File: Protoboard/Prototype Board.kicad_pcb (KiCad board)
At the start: 2 copper layers, 99.1 x 99.1 mm, 433 parts, among them J1 Conn_01x01, J10 Conn_01x01, J100 Connectable_Pad_Group_01x04, J101 Connectable_Pad_Group_01x04, J102 Connectable_Pad_Group_01x04, J103 Connectable_Pad_Group_01x04, J104 Connectable_Pad_Group_01x04, J105 Connectable_Pad_Group_01x04, J106 Connectable_Pad_Group_01x04, J107 Connectable_Pad_Group_01x04, J108 Connectable_Pad_Group_01x04, J109 Connectable_Pad_Group_01x04, J11 Conn_01x01, J110 Connectable_Pad_Group_01x04, J111 Connectable_Pad_Group_01x04, J112 Connectable_Pad_Group_01x04, J113 Connectable_Pad_Group_01x04, J114 Connectable_Pad_Group_01x04, J115 Connectable_Pad_Group_01x04, J116 Connectable_Pad_Group_01x04, J117 Connectable_Pad_Group_01x04, J118 Connectable_Pad_Group_01x04, J119 Connectable_Pad_Group_01x04, J12 Conn_01x01, J120 Connectable_Pad_Group_01x04, J121 Connectable_Pad_Group_01x04, J122 Connectable_Pad_Group_01x04, J123 Connectable_Pad_Group_01x04, J124 Connectable_Pad_Group_01x04, J125 Connectable_Pad_Group_01x04, J126 Connectable_Pad_Group_01x04, J13 Conn_01x01, J133 Conn_01x03_Male, J134 Conn_01x03_Male, J135 Connectable_Pad_Group_01x04, J136 Connectable_Pad_Group_01x04, J137 Connectable_Pad_Group_01x04, J138 Connectable_Pad_Group_01x04, J139 Connectable_Pad_Group_01x04, J14 Conn_01x01, J140 Connectable_Pad_Group_01x04, J141 Connectable_Pad_Group_01x04, J142 Connectable_Pad_Group_01x04, J143 Connectable_Pad_Group_01x04, J144 Connectable_Pad_Group_01x04, J145 Connectable_Pad_Group_01x04, J146 Connectable_Pad_Group_01x04, J147 Connectable_Pad_Group_01x04, J148 Connectable_Pad_Group_01x04, J149 Connectable_Pad_Group_01x04, J15 Conn_01x01, J150 Connectable_Pad_Group_01x04, J151 Connectable_Pad_Group_01x04, J152 Connectable_Pad_Group_01x04, J153 Connectable_Pad_Group_01x04, J154 Connectable_Pad_Group_01x04, J155 Connectable_Pad_Group_01x04, J156 Connectable_Pad_Group_01x04, J157 Connectable_Pad_Group_01x04, J158 Connectable_Pad_Group_01x04, J159 Connectable_Pad_Group_01x04, J16 Conn_01x01, J160 Connectable_Pad_Group_01x04, J161 Connectable_Pad_Group_01x04, J162 Connectable_Pad_Group_01x04, J163 Connectable_Pad_Group_01x04, J164 Connectable_Pad_Group_01x04, J165 Conn_01x03_Male, J166 Conn_01x03_Male, J17 Connectable_Pad_Group_01x04, J18 Connectable_Pad_Group_01x04, J19 Connectable_Pad_Group_01x04, J2 Conn_01x01, J20 Connectable_Pad_Group_01x04, J21 Connectable_Pad_Group_01x04, J22 Connectable_Pad_Group_01x04, J23 Connectable_Pad_Group_01x04, J24 Connectable_Pad_Group_01x04, J25 Connectable_Pad_Group_01x04, J26 Connectable_Pad_Group_01x04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

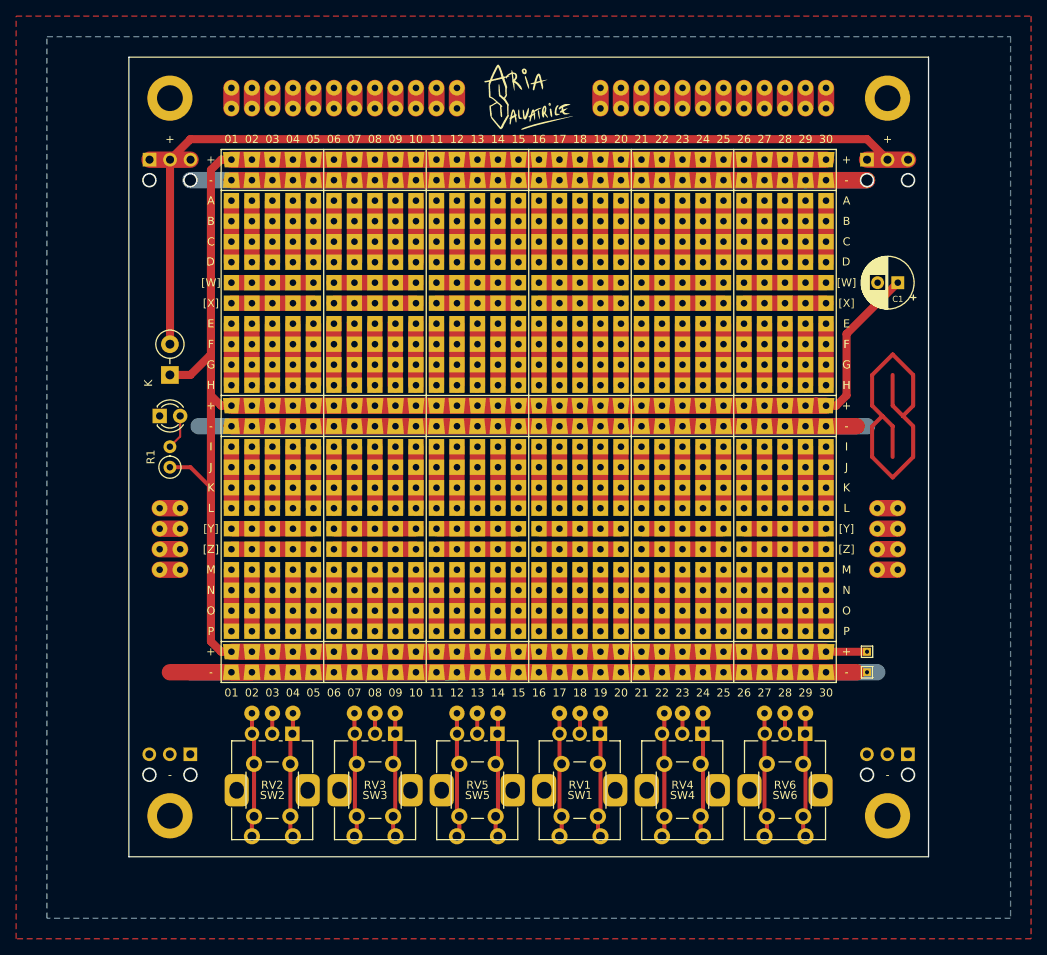
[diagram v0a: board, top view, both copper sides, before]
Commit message: Protoboard Rev2 ready soon, needs checking
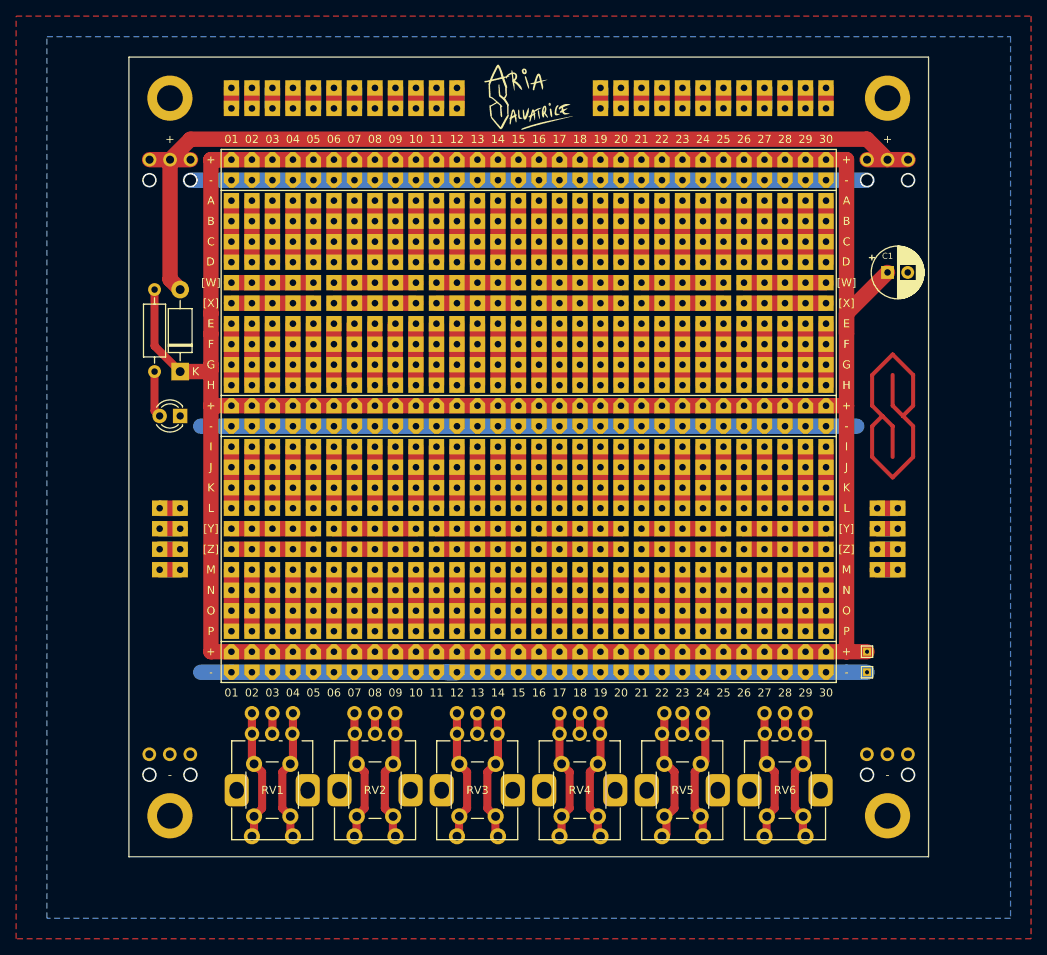
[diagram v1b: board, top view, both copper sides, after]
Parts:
- removed the J167 at (170.2, 43.2)
- removed J168, J169, J170, J171, J172, J173, J193, J194, J195, J196, J197, J198, J214, J215, J216, J217, J218, J219, J220, J221, J222, J223, J224, J225, J226, J227, J228, J229, J230, J231, J232, J233, J234, J235, J236, J237, J238, J239, J240, J241, J242, J243, J244, J245, J246, J247, J248, J249, J250, J251, J252, J253, J254, J255, J256, J257, J258, J259, J260, J261, J262, J263, J264, J265, J266, J267, J268, J269, J270, J271, J272, J273, J274, J275, J276, J277, J278, J279, J280, J281, J282, J283, J284, J285, J286, J287, J288, J289, J290, J291, J292, J293, J294, J295, J296, J297, J298, J299, J300, J301, J302, J303, J304, J305, J306, J307, J308, J309, J310, J311, J312, J313, J314, J315, J316, J317, J318, J319, J320, J321, J322, J323, J324, J325, J326, J327, J328, J329, J330, J331, J332, J333, J334, J335, J336, J337, J338, J339, J340, J341, J342, J343, J344, J345, J346: ~, ao_tht:Perf_Board_Hole
- removed the J174 at (167.6, 43.2)
- removed the J175 at (127.0, 43.2)
- removed the J176 at (142.2, 43.2)
- removed the J177 at (114.3, 43.2)
- removed the J178 at (116.8, 43.2)
- removed the J179 at (149.9, 43.2)
- removed the J180 at (106.7, 43.2)
- removed the J181 at (147.3, 43.2)
- removed the J182 at (172.7, 43.2)
- removed the J183 at (154.9, 43.2)
- removed the J184 at (124.5, 43.2)
- removed the J185 at (119.4, 43.2)
- removed the J186 at (144.8, 43.2)
- removed the J187 at (109.2, 43.2)
- removed the J188 at (152.4, 43.2)
- removed the J189 at (139.7, 43.2)
- removed the J190 at (162.6, 43.2)
- removed the J191 at (132.1, 43.2)
- removed the J192 at (160.0, 43.2)
- removed the J199 at (165.1, 45.7)
- removed the J200 at (137.2, 45.7)
- removed the J201 at (116.8, 45.7)
- removed the J202 at (144.8, 45.7)
- removed the J203 at (127.0, 45.7)
- removed the J204 at (157.5, 45.7)
- removed the J205 at (149.9, 45.7)
- removed the J206 at (124.5, 45.7)
- removed the J207 at (114.3, 45.7)
- removed the J208 at (175.3, 45.7)
- removed the J209 at (104.1, 45.7)
- removed the J210 at (139.7, 45.7)
- removed the J211 at (106.7, 45.7)
- removed the J212 at (160.0, 45.7)
- removed the J213 at (109.2, 45.7)
- removed the REF** at (177.8, 34.3)
- removed the REF** at (132.1, 34.3)
- removed the REF** at (95.2, 91.4)
- removed the REF** at (121.9, 36.8)
- removed the REF** at (152.4, 34.3)
- removed the REF** at (184.2, 94.0)
- removed the REF** at (97.8, 91.4)
- removed the REF** at (167.6, 36.8)
- removed the REF** at (97.8, 94.0)
- removed the REF** at (152.4, 36.8)
- removed the REF** at (114.3, 34.3)
- removed the REF** at (160.0, 34.3)
- removed the REF** at (184.2, 88.9)
- removed the REF** at (175.3, 36.8)
- removed the REF** at (172.7, 34.3)
- removed the REF** at (95.2, 86.4)
- removed the REF** at (170.2, 34.3)
- removed the REF** at (129.5, 34.3)
- removed the REF** at (175.3, 34.3)
- removed the REF** at (154.9, 34.3)
- removed the REF** at (109.2, 34.3)
- removed the REF** at (111.8, 34.3)
- removed the REF** at (119.4, 34.3)
- removed the REF** at (116.8, 34.3)
- removed the REF** at (165.1, 36.8)
- removed the REF** at (184.2, 91.4)
- removed the REF** at (119.4, 36.8)
- removed the REF** at (157.5, 36.8)
- removed the REF** at (160.0, 36.8)
- removed the REF** at (186.7, 94.0)
- removed the REF** at (170.2, 36.8)
- removed the REF** at (154.9, 36.8)
- removed the REF** at (132.1, 36.8)
- removed the REF** at (124.5, 36.8)
- removed the REF** at (95.2, 88.9)
- removed the REF** at (127.0, 36.8)
- removed the REF** at (172.7, 36.8)
- removed the REF** at (149.9, 34.3)
- removed the REF** at (111.8, 36.8)
- removed the REF** at (186.7, 91.4)
- removed the REF** at (97.8, 86.4)
- removed the REF** at (106.7, 34.3)
- removed the REF** at (129.5, 36.8)
- removed the REF** at (177.8, 36.8)
- removed the REF** at (186.7, 86.4)
- removed the REF** at (116.8, 36.8)
- removed the REF** at (97.8, 88.9)
- removed the REF** at (186.7, 88.9)
- removed the REF** at (104.1, 34.3)
- removed the REF** at (109.2, 36.8)
- removed the REF** at (124.5, 34.3)
- removed the REF** at (106.7, 36.8)
- removed the REF** at (167.6, 34.3)
- removed the REF** at (104.1, 36.8)
- removed the REF** at (95.2, 94.0)
- removed the REF** at (121.9, 34.3)
- removed the REF** at (127.0, 34.3)
- removed the REF** at (114.3, 36.8)
- removed the REF** at (157.5, 34.3)
- removed the REF** at (184.2, 86.4)
- removed the REF** at (162.6, 34.3)
- removed the REF** at (165.1, 34.3)
- removed the REF** at (149.9, 36.8)
- removed the REF** at (162.6, 36.8)
- added J1: Connectable_Pad_Group_01x02, Protoboard:Connectable_Pad_Group_01x02, F.Cu at (97.8, 86.4)
- added J103: Connectable_Pad_Group_01x02, Protoboard:Connectable_Pad_Group_01x02, F.Cu at (157.5, 34.3)
- added J11: Power_Rail_30, Protoboard:Power_Rail_30, F.Cu at (104.1, 43.2)
- added J112: Connectable_Pad_Group_01x02, Protoboard:Connectable_Pad_Group_01x02, F.Cu at (160.0, 34.3)
- added J113: Connectable_Pad_Group_01x02, Protoboard:Connectable_Pad_Group_01x02, F.Cu at (162.6, 34.3)
- added J124: Connectable_Pad_Group_01x02, Protoboard:Connectable_Pad_Group_01x02, F.Cu at (165.1, 34.3)
- added J129: Connectable_Pad_Group_01x02, Protoboard:Connectable_Pad_Group_01x02, F.Cu at (167.6, 34.3)
- added J13: Power_Rail_30, Protoboard:Power_Rail_30, F.Cu at (104.1, 73.7)
- added J134: Connectable_Pad_Group_01x02, Protoboard:Connectable_Pad_Group_01x02, F.Cu at (170.2, 34.3)
- added J139: Connectable_Pad_Group_01x02, Protoboard:Connectable_Pad_Group_01x02, F.Cu at (172.7, 34.3)
- added J146: Connectable_Pad_Group_01x02, Protoboard:Connectable_Pad_Group_01x02, F.Cu at (175.3, 34.3)
- added J15: Power_Rail_30, Protoboard:Power_Rail_30, F.Cu at (104.1, 104.1)
- added J151: Connectable_Pad_Group_01x02, Protoboard:Connectable_Pad_Group_01x02, F.Cu at (186.7, 86.4)
- added J152: Connectable_Pad_Group_01x02, Protoboard:Connectable_Pad_Group_01x02, F.Cu at (186.7, 88.9)
- added J153: Connectable_Pad_Group_01x02, Protoboard:Connectable_Pad_Group_01x02, F.Cu at (186.7, 91.4)
- added J154: Connectable_Pad_Group_01x02, Protoboard:Connectable_Pad_Group_01x02, F.Cu at (186.7, 94.0)
- added J159: Connectable_Pad_Group_01x02, Protoboard:Connectable_Pad_Group_01x02, F.Cu at (177.8, 34.3)
- added J16: Connectable_Pad_Group_01x02, Protoboard:Connectable_Pad_Group_01x02, F.Cu at (109.2, 34.3)
- added J2: Connectable_Pad_Group_01x02, Protoboard:Connectable_Pad_Group_01x02, F.Cu at (97.8, 88.9)
- added J25: Connectable_Pad_Group_01x02, Protoboard:Connectable_Pad_Group_01x02, F.Cu at (111.8, 34.3)
- added J3: Connectable_Pad_Group_01x02, Protoboard:Connectable_Pad_Group_01x02, F.Cu at (97.8, 91.4)
- added J30: Connectable_Pad_Group_01x02, Protoboard:Connectable_Pad_Group_01x02, F.Cu at (114.3, 34.3)
- added J35: Connectable_Pad_Group_01x02, Protoboard:Connectable_Pad_Group_01x02, F.Cu at (116.8, 34.3)
- added J4: Connectable_Pad_Group_01x02, Protoboard:Connectable_Pad_Group_01x02, F.Cu at (97.8, 94.0)
- added J42: Connectable_Pad_Group_01x02, Protoboard:Connectable_Pad_Group_01x02, F.Cu at (119.4, 34.3)
- added J47: Connectable_Pad_Group_01x02, Protoboard:Connectable_Pad_Group_01x02, F.Cu at (121.9, 34.3)
- added J5: Connectable_Pad_Group_01x02, Protoboard:Connectable_Pad_Group_01x02, F.Cu at (104.1, 34.3)
- added J56: Connectable_Pad_Group_01x02, Protoboard:Connectable_Pad_Group_01x02, F.Cu at (124.5, 34.3)
- added J6: Connectable_Pad_Group_01x02, Protoboard:Connectable_Pad_Group_01x02, F.Cu at (106.7, 34.3)
- added J61: Connectable_Pad_Group_01x02, Protoboard:Connectable_Pad_Group_01x02, F.Cu at (127.0, 34.3)
- added J62: Connectable_Pad_Group_01x02, Protoboard:Connectable_Pad_Group_01x02, F.Cu at (129.5, 34.3)
- added J73: Connectable_Pad_Group_01x02, Protoboard:Connectable_Pad_Group_01x02, F.Cu at (132.1, 34.3)
- added J86: Connectable_Pad_Group_01x02, Protoboard:Connectable_Pad_Group_01x02, F.Cu at (149.9, 34.3)
- added J91: Connectable_Pad_Group_01x02, Protoboard:Connectable_Pad_Group_01x02, F.Cu at (152.4, 34.3)
- added J98: Connectable_Pad_Group_01x02, Protoboard:Connectable_Pad_Group_01x02, F.Cu at (154.9, 34.3)
- D1: footprint Diode_THT:D_DO-41_SOD81_P3.81mm_Vertical_KathodeUp -> Diode_THT:D_DO-41_SOD81_P10.16mm_Horizontal
- R1: value 1K -> 4K7; footprint Resistor_THT:R_Axial_DIN0207_L6.3mm_D2.5mm_P2.54mm_Vertical -> Resistor_THT:R_Axial_DIN0207_L6.3mm_D2.5mm_P10.16mm_Horizontal
- moved R1 12.0 mm to (94.6, 69.4)
- moved D2 2.54 mm to (97.8, 74.9), turned to 180 degrees
- moved C1 1.80 mm to (185.4, 57.1), turned to 0 degrees
- moved D1 1.34 mm to (97.8, 69.4)
- renumbered J135 to J10, J80 to J100, J114 to J101, J152 to J102, J35 to J104, J81 to J105, J115 to J106, J153 to J107, J36 to J108, J82 to J109, J116 to J110, J154 to J111, J37 to J114, J83 to J115, J117 to J116, J155 to J117, J59 to J118, J131 to J119, J55 to J12, J38 to J120, J84 to J121, J118 to J122, J156 to J123, J39 to J125, J85 to J126, J119 to J127, J157 to J128, J40 to J130, J86 to J131, J120 to J132, J158 to J133, J41 to J135, J87 to J136, J121 to J137, J159 to J138, J127 to J14, J42 to J140, J88 to J141, J122 to J142, J160 to J143, J60 to J144, J132 to J145, J43 to J147, J89 to J148, J123 to J149, J161 to J150, J44 to J155, J90 to J156, J124 to J157, J162 to J158, J45 to J160, J91 to J161, J125 to J162, J46 to J164, J92 to J165, J126 to J166, J164 to J167, J18 to J17, J133 to J174, J165 to J175, J3 to J176, J9 to J177, J11 to J178, J47 to J179, J64 to J18, J51 to J180, J93 to J181, J4 to J182, J10 to J183, J12 to J184, J48 to J185, J52 to J186, J94 to J187, J6 to J188, J15 to J189, J98 to J19, J61 to J190, J134 to J191, J166 to J192, J1 to J199, J136 to J20, J7 to J200, J13 to J201, J49 to J202, J53 to J203, J95 to J204, J2 to J205, J8 to J206, J14 to J207, J50 to J208, J54 to J209, J19 to J21, J96 to J210, J5 to J211, J16 to J212, J62 to J213, J65 to J22, J99 to J23, J137 to J24, J20 to J26, J66 to J27, J100 to J28, J138 to J29, J21 to J31, J67 to J32, J101 to J33, J139 to J34, J22 to J36, J68 to J37, J102 to J38, J140 to J39, J56 to J40, J128 to J41, J23 to J43, J69 to J44, J103 to J45, J141 to J46, J24 to J48, J70 to J49, J104 to J50, J142 to J51, J25 to J52, J71 to J53, J105 to J54, J143 to J55, J26 to J57, J72 to J58, J106 to J59, J144 to J60, J27 to J63, J73 to J64, J107 to J65, J145 to J66, J57 to J67, J129 to J68, J28 to J69, J17 to J7, J74 to J70, J108 to J71, J146 to J72, J29 to J74, J109 to J76, J147 to J77, J30 to J78, J76 to J79, J63 to J8, J110 to J80, J148 to J81, J31 to J82, J77 to J83, J111 to J84, J149 to J85, J32 to J87, J78 to J88, J112 to J89, J97 to J9, J150 to J90, J58 to J92, J130 to J93, J33 to J94, J79 to J95, J113 to J96, J151 to J97, J34 to J99, RV2 to RV1, RV3 to RV2, RV5 to RV3, RV1 to RV4, RV4 to RV5, SW1 to SW10, SW4 to SW11, SW6 to SW12, SW2 to SW4, SW3 to SW5, SW5 to SW6
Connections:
- net Net-(D1-A) renamed /12V_Input
- R1 pad 1: +12V -> Net-(D2-A)
- R1 pad 2: Net-(D2-A) -> +12V
- RV1 pad MP: unconnected-(RV2-MountPin) -> (no net)
- RV2 pad MP: unconnected-(RV3-MountPin) -> (no net)
- RV3 pad MP: unconnected-(RV5-MountPin) -> (no net)
- RV4 pad MP: unconnected-(RV1-MountPin) -> (no net)
- RV5 pad MP: unconnected-(RV4-MountPin) -> (no net)
- RV6 pad MP: unconnected-(RV6-MountPin) -> (no net)
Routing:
- net GND: track 501.9 -> 248.9 mm
- net +12V: track 328.1 -> 388.3 mm
- net unconnected-(J8-Pad1): track 55.6 -> 7.62 mm
- net (no net): track 76.2 -> 48.0 mm
- net /12V_Input: track 124.0 -> 117.8 mm
- net unconnected-(J1-Pad1): track 0.00 -> 5.12 mm
- net unconnected-(J4-Pad1): track 0.00 -> 5.06 mm
- net unconnected-(J3-Pad1): track 0.00 -> 5.06 mm
- net unconnected-(J2-Pad1): track 0.00 -> 5.06 mm
- net unconnected-(J98-Pad1): track 0.00 -> 5.05 mm
- net unconnected-(J91-Pad1): track 0.00 -> 5.05 mm
- net unconnected-(J86-Pad1): track 0.00 -> 5.05 mm
- net unconnected-(J73-Pad1): track 0.00 -> 5.05 mm
- net unconnected-(J62-Pad1): track 0.00 -> 5.05 mm
- net unconnected-(J61-Pad1): track 0.00 -> 5.05 mm
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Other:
- board text added: "TODO LIST - Imported symbol to replace - Pass DRC (already pass the important parts)"
- board text removed: "TODO LIST - Bonus pads not on the schematic - Imported symbol to replace - Rotary encoder?? - Remake the cursed footprints - Redo schematic - Have 3D models - Can I fit in MORE knobs? - Use proper net width (sounds complicated) - Pass DRC lol"
